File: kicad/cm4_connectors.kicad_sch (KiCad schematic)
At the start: 9 parts, among them J3 Header-Male-2.54_2x3, J4 2541WV-2X12P, J5 Header-Male-2.54_1x3, J6 Header-Male-2.54_2x3, U10 74LVC1G07SE-7

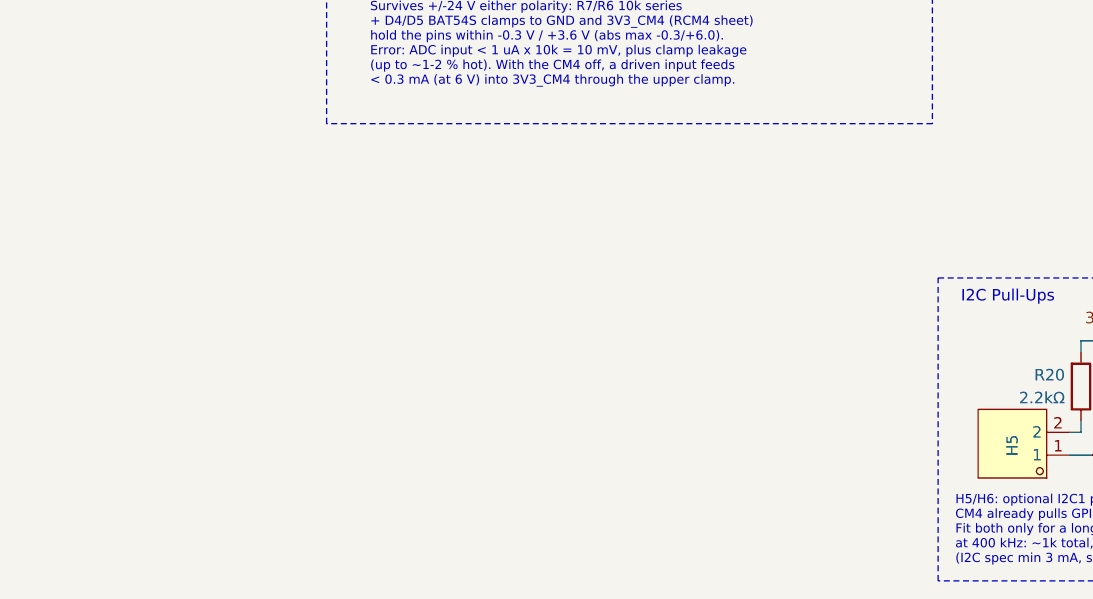
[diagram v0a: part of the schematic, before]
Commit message: Improved README
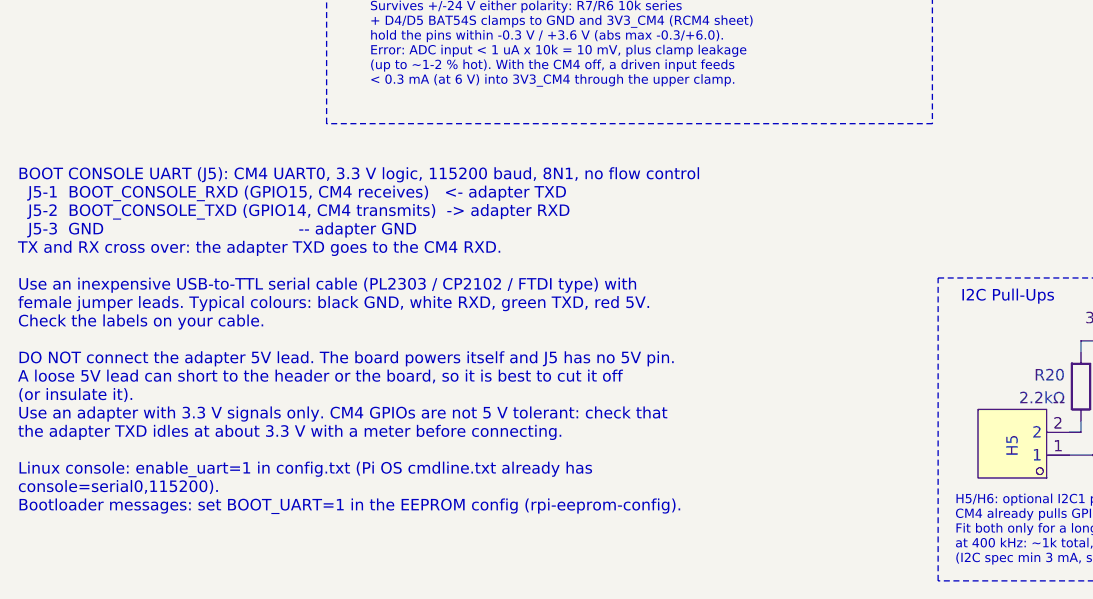
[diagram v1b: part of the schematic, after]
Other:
- note added: "BOOT CONSOLE UART (J5): CM4 UART0, 3.3 V logic, 115200 baud, 8N1, no flow control J5-1 BOOT_CONSOLE_RXD (GPIO15, CM4 receives) <- adapter TXD J5-2 BOOT_CONSOLE_TXD (GPIO14, CM4 transmits) -> adapter RXD J5-3 GND -- adapter GND TX and RX cross over: the adapter TXD goes to the CM4 RXD. Use an inexpensive USB-to-TTL serial cable (PL2303 / CP2102 / FTDI type) with female jumper leads. Typical colour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"
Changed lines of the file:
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@@
+		)
+	)
+	(text "BOOT CONSOLE UART (J5): CM4 UART0, 3.3 V logic, 115200 baud, 8N1, no flow control\n  J5-1  BOOT_CONSOLE_RXD (GPIO15, CM4 receives)   <- adapter TXD\n  J5-2  BOOT_CONSOLE_TXD (GPIO14, CM4 transmits)  -> adapter RXD\n  J5-3  GND                                       -- adapter GND\nTX and RX cross over: the adapter TXD goes to the CM4 RXD.\n\nUse an inexpensive USB-to-TTL serial cable (PL2303 / CP2102 / FTDI type) with\nfemale jumper leads. Typical colours: black GND, white RXD, green TXD, red 5V.\nCheck the labels on your cable.\n\nDO NOT connect the adapter 5V lead. The board powers itself and J5 has no 5V pin.\nA loose 5V lead can short to the header or the board, so it is best to cut it off\n(or insulate it).\nUse an adapter with 3.3 V signals only. CM4 GPIOs are not 5 V tolerant: check that\nthe adapter TXD idles at about 3.3 V with a meter before connecting.\n\nLinux console: enable_uart=1 in config.txt (Pi OS cmdline.txt already has\nconsole=serial0,115200).\nBootloader messages: set BOOT_UART=1 in the EEPROM config (rpi-eeprom-config)."
+		(exclude_from_sim no)
+		(at 16.51 147.32 0)
+		(effects
+			(font
+				(size 1.27 1.27)
+			)
+			(justify left top)
 		)
 	)
